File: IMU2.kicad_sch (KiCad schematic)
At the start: 3 parts, among them U3 262-BMI088

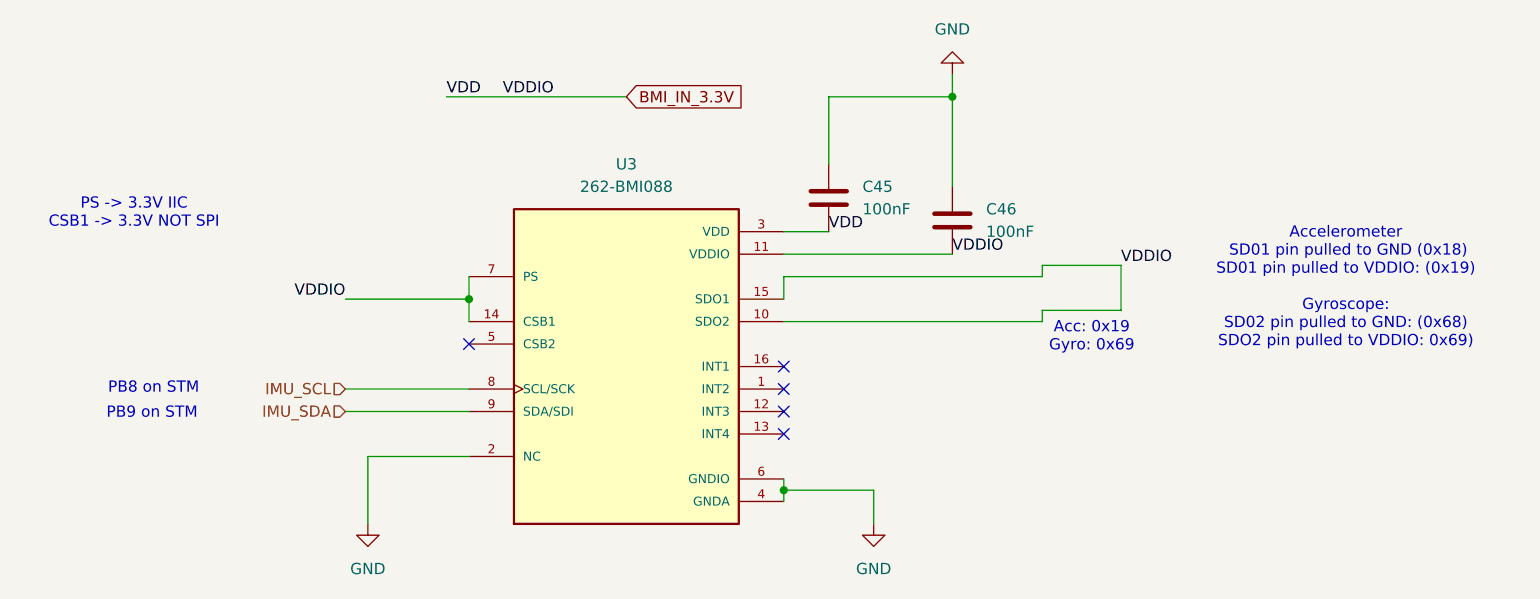
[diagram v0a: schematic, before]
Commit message: multiple chainges on PCB
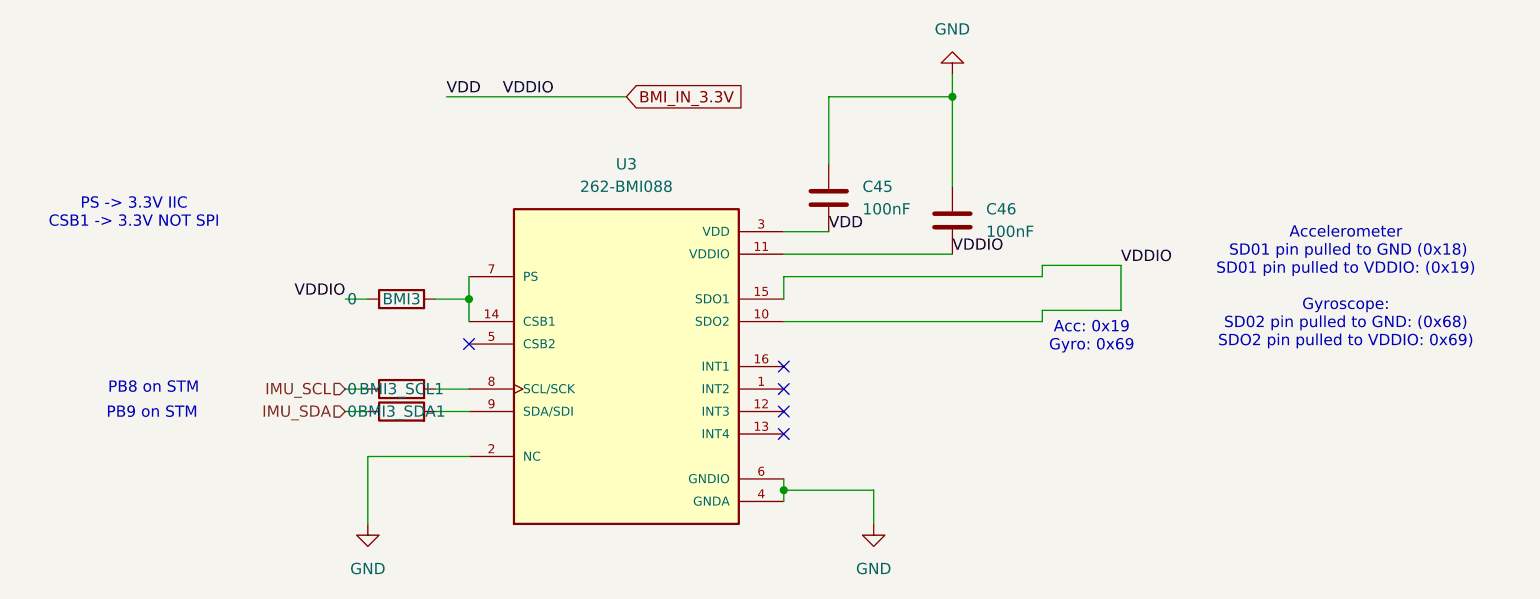
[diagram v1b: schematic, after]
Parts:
- added BMI3, BMI3_SCL1, BMI3_SDA1: 0, Resistor_SMD:R_0603_1608Metric, symbol #dzdb:g_res/R-0-0603
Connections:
- net BMI_IN_3.3V: now also BMI3.1; no longer U3.14 (CSB1), U3.7 (PS)
- net IMU_SCL: now also BMI3_SCL1.1; no longer U3.8 (SCL/SCK)
- net IMU_SDA: now also BMI3_SDA1.1; no longer U3.9 (SDA/SDI)
- new net: BMI3_SCL1.2, U3.8 (SCL/SCK)
- new net: BMI3.2, U3.14 (CSB1), U3.7 (PS)
- new net: BMI3_SDA1.2, U3.9 (SDA/SDI)
